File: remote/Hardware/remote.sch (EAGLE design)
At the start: 30 parts, among them IC1 TINY13-20PU

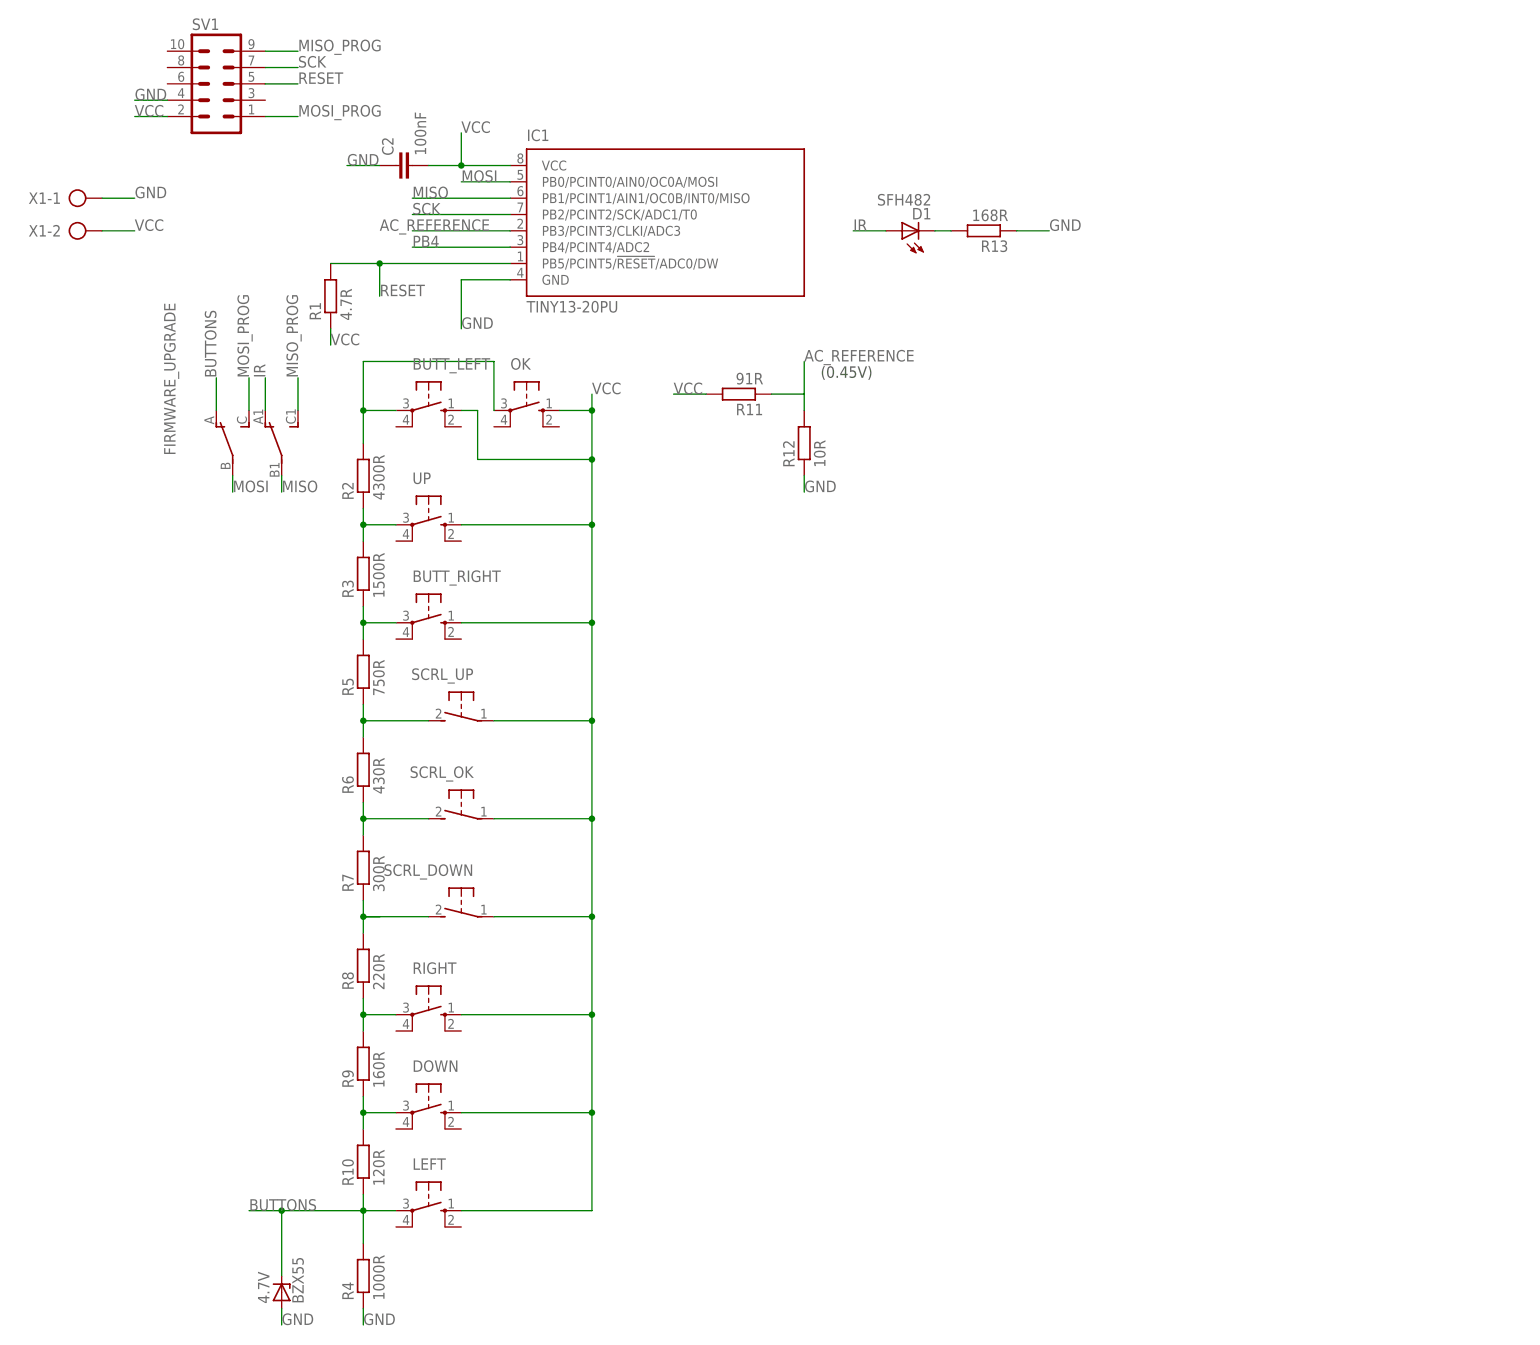
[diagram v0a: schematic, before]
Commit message: Naprawa Plytki pilota, gotowe do termotransferu
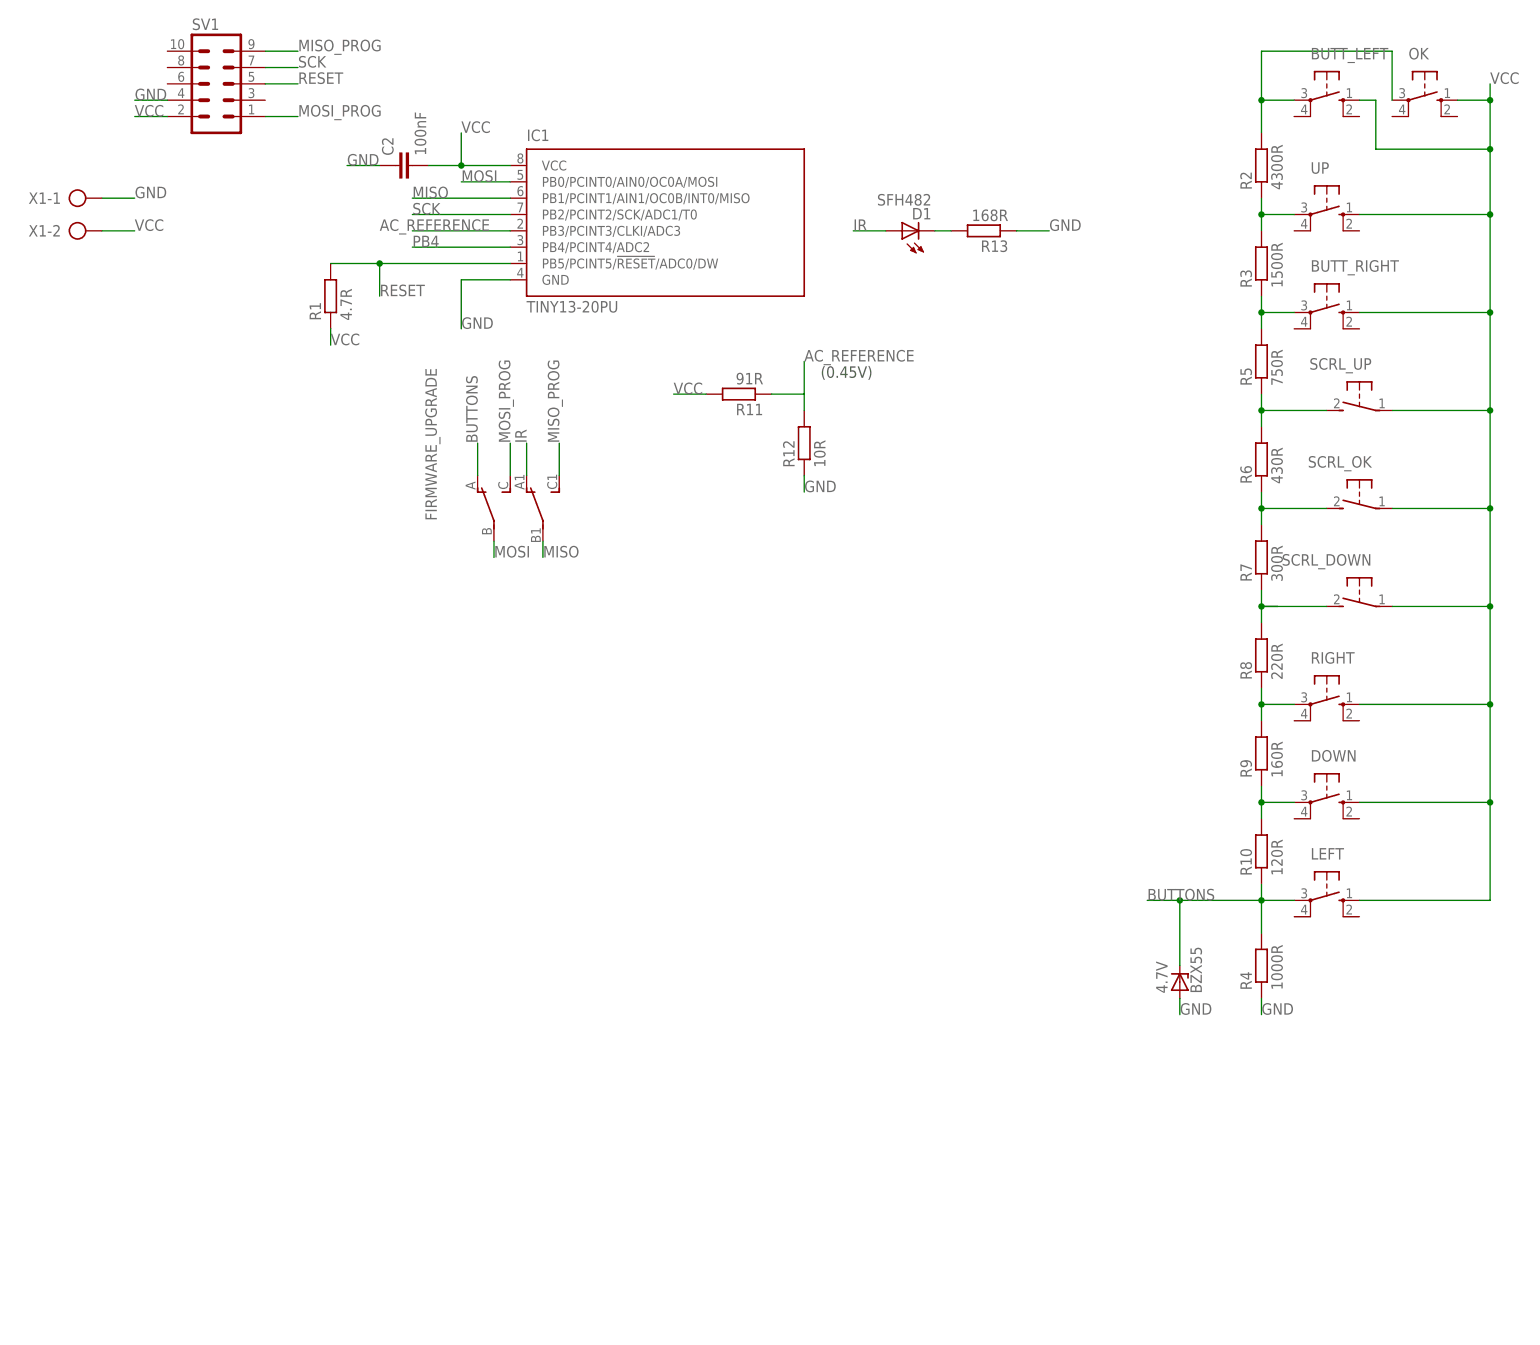
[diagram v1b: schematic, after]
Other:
- moved on the sheet: 4.7V, BUTT_LEFT, BUTT_RIGHT, DOWN, FIRMWARE_UPGRADE, LEFT, OK, R10, R2, R3, R4, R5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
